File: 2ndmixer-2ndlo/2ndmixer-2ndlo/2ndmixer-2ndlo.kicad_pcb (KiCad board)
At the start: 2 copper layers, 72.4 x 49.5 mm, 57 parts, among them J201 Coax Solder Point, J202 Conn_01x02, J203 Coax Solder Point, Q201 2N5179, Q202 2N5179, T201 Bifilar_Transformer, U201 MAV-11, U202 TUF-1H+, Y201 100MHz

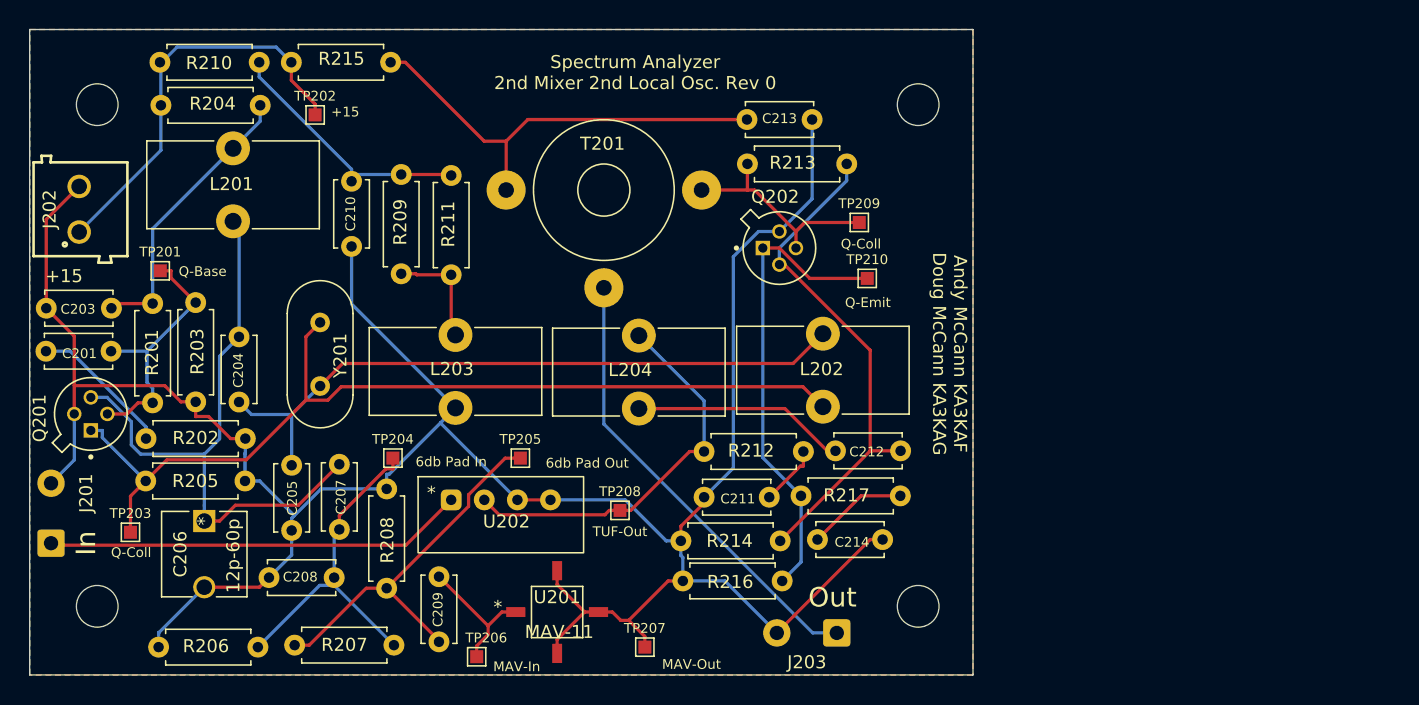
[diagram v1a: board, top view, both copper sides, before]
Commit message: 2ndmixer-2ndlo rev 1
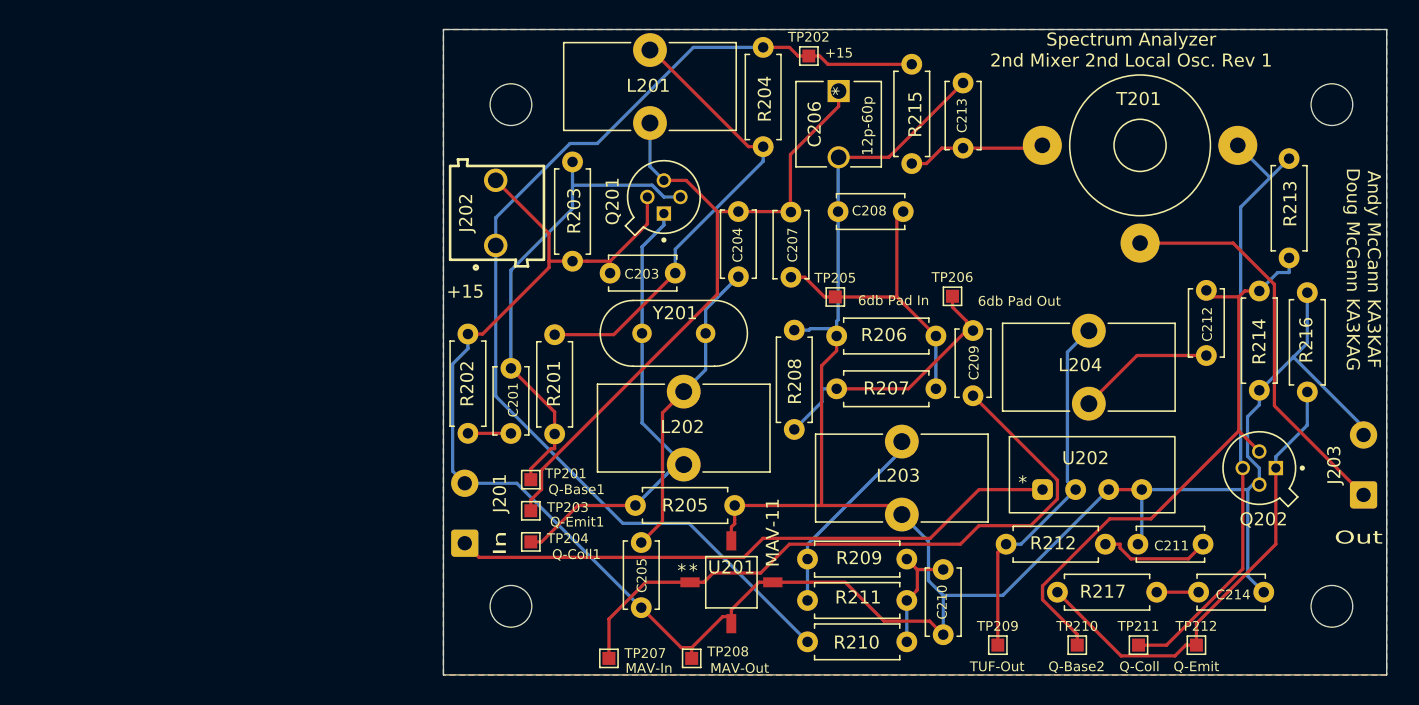
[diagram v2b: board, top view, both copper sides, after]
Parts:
- added TP203: Q-Emit1, TestPoint:TestPoint_Pad_1.0x1.0mm, F.Cu at (141.1, 112.2)
- added TP210: Q-Base2, TestPoint:TestPoint_Pad_1.0x1.0mm, F.Cu at (183.1, 122.5)
- TP201: value Q-Base -> Q-Base1
- TP204: renamed from TP203; value Q-Coll -> Q-Coll1
- TP211: renamed from TP209; value Q-Coll -> Q-Coll2
- TP212: renamed from TP210; value Q-Emit -> Q-Emit2
- U202: footprint 2ndmixer-2ndlo:TUF-1H -> spectrum_analyzer:TUF-1H
- moved R210 66.7 mm to (162.4, 122.2)
- moved C206 58.8 mm to (164.7, 80.0)
- moved R206 57.3 mm to (172.2, 98.8)
- moved C210 54.3 mm to (172.8, 116.7)
- moved C208 51.9 mm to (169.7, 89.2)
- moved R209 48.8 mm to (170.0, 115.9), turned to 180 degrees
- moved R211 47.8 mm to (170.0, 119.0), turned to 180 degrees
- moved R215 47.6 mm to (170.4, 77.9), turned to -90 degrees
- moved C209 47.4 mm to (175.1, 98.3), turned to -90 degrees
- moved Q201 47.0 mm to (151.3, 88.1)
- moved R204 46.4 mm to (159.0, 76.6), turned to -90 degrees
- moved R207 46.0 mm to (172.2, 102.8)
- moved U202 45.4 mm to (180.4, 110.5)
- moved C203 43.4 mm to (152.2, 93.9)
- moved R216 42.8 mm to (200.7, 103.0), turned to 90 degrees
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- renumbered TP204 to TP205, TP205 to TP206, TP206 to TP207, TP207 to TP208, TP208 to TP209
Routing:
- net /+15: track 31.5 -> 83.3 mm
- net Net-(U201-RF_In): track 10.6 -> 51.9 mm
- net Net-(L202-Pad2): track 72.6 -> 35.3 mm
- net Net-(Q202-Pad3): track 17.0 -> 47.0 mm
- net Net-(C204-Pad2): track 51.7 -> 23.5 mm
- net Net-(C213-Pad2): track 34.3 -> 10.6 mm
- net GND: track 200.6 -> 222.8 mm
- net Net-(C201-Pad1): track 20.1 -> 37.3 mm
- net Net-(J201-In): track 32.2 -> 46.9 mm
- net Net-(C203-Pad1): track 21.9 -> 35.5 mm
- net Net-(C210-Pad1): track 19.7 -> 9.01 mm
- net Net-(C209-Pad1): track 29.6 -> 20.5 mm
- net Net-(C201-Pad2): track 11.0 -> 3.31 mm
- net Net-(C204-Pad1): track 48.0 -> 55.3 mm
- net Net-(C212-Pad2): track 39.4 -> 46.6 mm
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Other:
- board text added: "Spectrum Analyzer 2nd Mixer 2nd Local Osc. Rev 1"
- board text removed: "Spectrum Analyzer 2nd Mixer 2nd Local Osc. Rev 0"
